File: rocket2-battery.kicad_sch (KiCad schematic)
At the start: 58 parts, among them J1 Conn_01x07, J2 SMA, J3 ARM Cortex Debug, P1 PAD_SMD, P2 PAD_SMD, P3 PAD_SMD, P4 PAD_SMD, P5 PAD_SMD, P6 PAD_SMD, P7 PAD_SMD, Q1 NMOS, Q2 NMOS, Q3 PMOS, Q4 PMOS, Q5 NMOS, Q6 NMOS, Q7 PMOS, Q8 PMOS, U1 3V3 LDO, Y1 16MHz

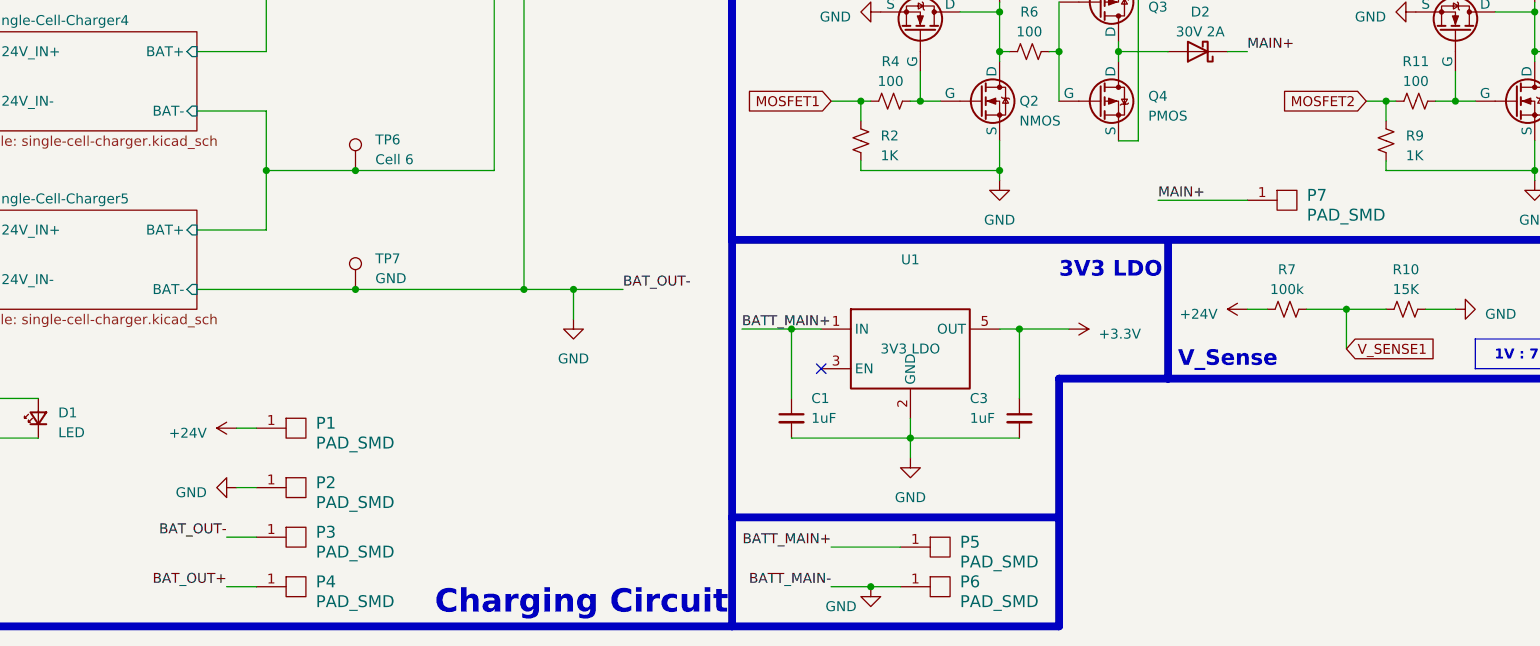
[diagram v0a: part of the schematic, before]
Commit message: Almost done routing
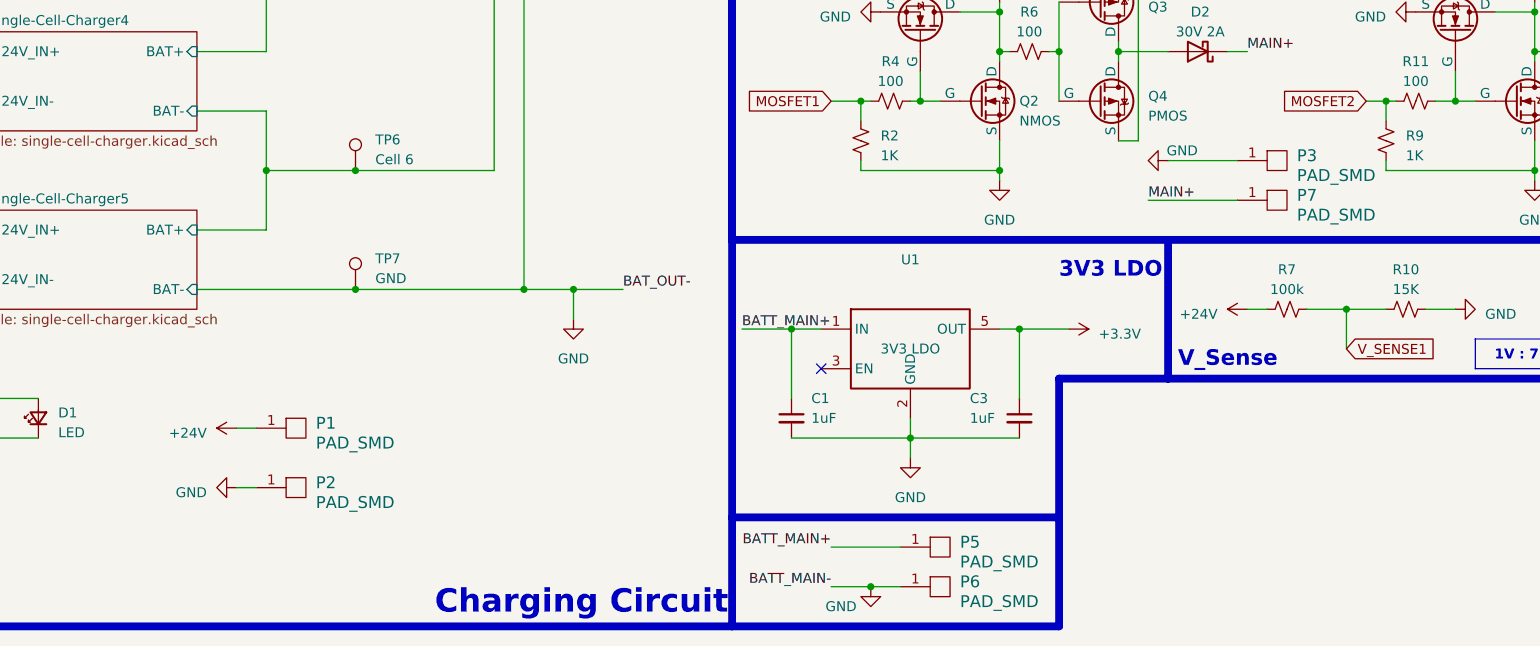
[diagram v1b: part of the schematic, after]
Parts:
- removed P4: PAD_SMD, TestPoint:TestPoint_Pad_2.0x2.0mm, symbol pkl_misc:PAD_SMD
- R8: footprint Resistor_SMD:R_0603_1608Metric -> Resistor_SMD:R_0603_1608Metric_Pad0.98x0.95mm_HandSolder
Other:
- moved on the sheet: P7
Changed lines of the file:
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@@
     (stroke (width 0) (type default))
   )
-  (wire (pts (xy 189.23 142.24) (xy 200.66 142.24))
+  (wire (pts (xy 187.96 142.24) (xy 199.39 142.24))
     (stroke (width 0) (type default))
   )
@@
     (stroke (width 0) (type default))
   )
-  (wire (pts (xy 69.85 185.42) (xy 73.66 185.42))
-    (stroke (width 0) (type default))
-  )
   (wire (pts (xy 255.27 95.25) (xy 257.81 95.25))
     (stroke (width 0) (type default))
@@
     (stroke (width 0) (type default))
   )
+  (wire (pts (xy 190.5 137.16) (xy 199.39 137.16))
+    (stroke (width 0) (type default))
+  )
   (wire (pts (xy 147.32 191.77) (xy 152.4 191.77))
     (stroke (width 0) (type default))
@@
     (stroke (width 0) (type default))
   )
-  (wire (pts (xy 69.85 191.77) (xy 73.66 191.77))
-    (stroke (width 0) (type default))
-  )
   (wire (pts (xy 208.28 156.21) (xy 213.36 156.21))
     (stroke (width 0) (type default))
@@
     (effects (font (size 1.27 1.27)) (justify left bottom))
   )
-  (label "MAIN+" (at 189.23 142.24 0) (fields_autoplaced)
+  (label "MAIN+" (at 187.96 142.24 0) (fields_autoplaced)
     (effects (font (size 1.27 1.27)) (justify left bottom))
   )
@@
     (effects (font (size 1.27 1.27)) (justify right bottom))
   )
-  (label "BAT_OUT-" (at 69.85 185.42 180) (fields_autoplaced)
-    (effects (font (size 1.27 1.27)) (justify right bottom))
-  )
   (label "BATT_MAIN+" (at 237.49 109.22 0) (fields_autoplaced)
     (effects (font (size 1.27 1.27)) (justify left bottom))
   )
-  (label "BAT_OUT+" (at 69.85 191.77 180) (fields_autoplaced)
-    (effects (font (size 1.27 1.27)) (justify right bottom))
-  )
   (label "BATT_MAIN+" (at 135.89 158.75 0) (fields_autoplaced)
     (effects (font (size 1.27 1.27)) (justify left bottom))
@@
     )
   )
+  (symbol (lib_id "power:GND") (at 190.5 137.16 270) (unit 1)
+    (in_bom yes) (on_board yes) (dnp no)
+    (property "Reference" "#PWR044" (at 184.15 137.16 0)
+      (effects (font (size 1.27 1.27)) hide)
+    )
+    (property "Value" "GND" (at 194.31 135.89 90)
+      (effects (font (size 1.27 1.27)) (justify right))
+    )
+    (property "Footprint" "" (at 190.5 137.16 0)
+      (effects (font (size 1.27 1.27)) hide)
+    )
+    (property "Datasheet" "" (at 190.5 137.16 0)
+      (effects (font (size 1.27 1.27)) hide)
+    )
+    (pin "1")
+    (instances
+      (project "rocket2-battery"
+        (path "/453543af-7e3c-49a0-a644-4bd49c4f86f8"
+          (reference "#PWR044") (unit 1)
+        )
+      )
+    )
+  )
   (symbol (lib_id "Device:LED_Small") (at 222.25 62.23 180) (unit 1)
     (in_bom yes) (on_board yes) (dnp no)
@@
     )
   )
-  (symbol (lib_id "pkl_misc:PAD_SMD") (at 78.74 191.77 0) (unit 1)
-    (in_bom yes) (on_board yes) (dnp no) (fields_autoplaced)
-    (property "Reference" "P4" (at 81.28 191.135 0)
-      (effects (font (size 1.524 1.524)) (justify left))
-    )
-    (property "Value" "PAD_SMD" (at 81.28 193.675 0)
-      (effects (font (size 1.524 1.524)) (justify left))
-    )
-    (property "Footprint" "TestPoint:TestPoint_Pad_2.0x2.0mm" (at 78.74 198.12 0)
-      (effects (font (size 1.524 1.524)) hide)
-    )
-    (property "Datasheet" "~" (at 78.74 195.58 0)
-      (effects (font (size 1.524 1.524)))
-    )
-    (property "Manufacturer" "Generic" (at 78.74 191.77 0)
-      (effects (font (size 1.27 1.27)) hide)
-    )
-    (pin "1")
-    (instances
-      (project "rocket2-battery"
-        (path "/453543af-7e3c-49a0-a644-4bd49c4f86f8"
-          (reference "P4") (unit 1)
-        )
-      )
-    )
-  )
   (symbol (lib_id "Device:C_Small") (at 210.82 22.86 0) (unit 1)
     (in_bom yes) (on_board yes) (dnp no)
@@
     )
   )
-  (symbol (lib_id "pkl_misc:PAD_SMD") (at 78.74 185.42 0) (unit 1)
-    (in_bom yes) (on_board yes) (dnp no) (fields_autoplaced)
-    (property "Reference" "P3" (at 81.28 184.785 0)
-      (effects (font (size 1.524 1.524)) (justify left))
-    )
-    (property "Value" "PAD_SMD" (at 81.28 187.325 0)
-      (effects (font (size 1.524 1.524)) (justify left))
-    )
-    (property "Footprint" "TestPoint:TestPoint_Pad_2.0x2.0mm" (at 78.74 191.77 0)
-      (effects (font (size 1.524 1.524)) hide)
-    )
-    (property "Datasheet" "~" (at 78.74 189.23 0)
-      (effects (font (size 1.524 1.524)))
-    )
-    (property "Manufacturer" "Generic" (at 78.74 185.42 0)
-      (effects (font (size 1.27 1.27)) hide)
-    )
-    (pin "1")
-    (instances
-      (project "rocket2-battery"
-        (path "/453543af-7e3c-49a0-a644-4bd49c4f86f8"
-          (reference "P3") (unit 1)
-        )
-      )
-    )
-  )
   (symbol (lib_id "power:+3.3V") (at 275.59 58.42 0) (unit 1)
     (in_bom yes) (on_board yes) (dnp no)
@@
     )
   )
+  (symbol (lib_id "pkl_misc:PAD_SMD") (at 204.47 137.16 0) (unit 1)
+    (in_bom yes) (on_board yes) (dnp no) (fields_autoplaced)
+    (property "Reference" "P3" (at 207.01 136.525 0)
+      (effects (font (size 1.524 1.524)) (justify left))
+    )
+    (property "Value" "PAD_SMD" (at 207.01 139.065 0)
+      (effects (font (size 1.524 1.524)) (justify left))
+    )
+    (property "Footprint" "TestPoint:TestPoint_Pad_2.0x2.0mm" (at 204.47 143.51 0)
+      (effects (font (size 1.524 1.524)) hide)
+    )
+    (property "Datasheet" "~" (at 204.47 140.97 0)
+      (effects (font (size 1.524 1.524)))
+    )
+    (property "Manufacturer" "Generic" (at 204.47 137.16 0)
+      (effects (font (size 1.27 1.27)) hide)
+    )
+    (pin "1")
+    (instances
+      (project "rocket2-battery"
+        (path "/453543af-7e3c-49a0-a644-4bd49c4f86f8"
+          (reference "P3") (unit 1)
+        )
+      )
+    )
+  )
   (symbol (lib_id "Connector:Conn_Coaxial") (at 232.41 93.98 90) (mirror x) (unit 1)
     (in_bom yes) (on_board yes) (dnp no)
@@
     )
   )
-  (symbol (lib_id "pkl_misc:PAD_SMD") (at 205.74 142.24 0) (unit 1)
+  (symbol (lib_id "pkl_misc:PAD_SMD") (at 204.47 142.24 0) (unit 1)
     (in_bom yes) (on_board yes) (dnp no) (fields_autoplaced)
-    (property "Reference" "P7" (at 208.28 141.605 0)
+    (property "Reference" "P7" (at 207.01 141.605 0)
       (effects (font (size 1.524 1.524)) (justify left))
     )
-    (property "Value" "PAD_SMD" (at 208.28 144.145 0)
+    (property "Value" "PAD_SMD" (at 207.01 144.145 0)
       (effects (font (size 1.524 1.524)) (justify left))
     )
-    (property "Footprint" "TestPoint:TestPoint_Pad_2.0x2.0mm" (at 205.74 148.59 0)
+    (property "Footprint" "TestPoint:TestPoint_Pad_2.0x2.0mm" (at 204.47 148.59 0)
       (effects (font (size 1.524 1.524)) hide)
     )
-    (property "Datasheet" "~" (at 205.74 146.05 0)
+    (property "Datasheet" "~" (at 204.47 146.05 0)
       (effects (font (size 1.524 1.524)))
     )
-    (property "Manufacturer" "Generic" (at 205.74 142.24 0)
+    (property "Manufacturer" "Generic" (at 204.47 142.24 0)
       (effects (font (size 1.27 1.27)) hide)
     )
@@
       (effects (font (size 1.27 1.27)))
     )
-    (property "Footprint" "Resistor_SMD:R_0603_1608Metric" (at 213.36 62.23 0)
+    (property "Footprint" "Resistor_SMD:R_0603_1608Metric_Pad0.98x0.95mm_HandSolder" (at 213.36 62.23 0)
       (effects (font (size 1.27 1.27)) hide)
     )

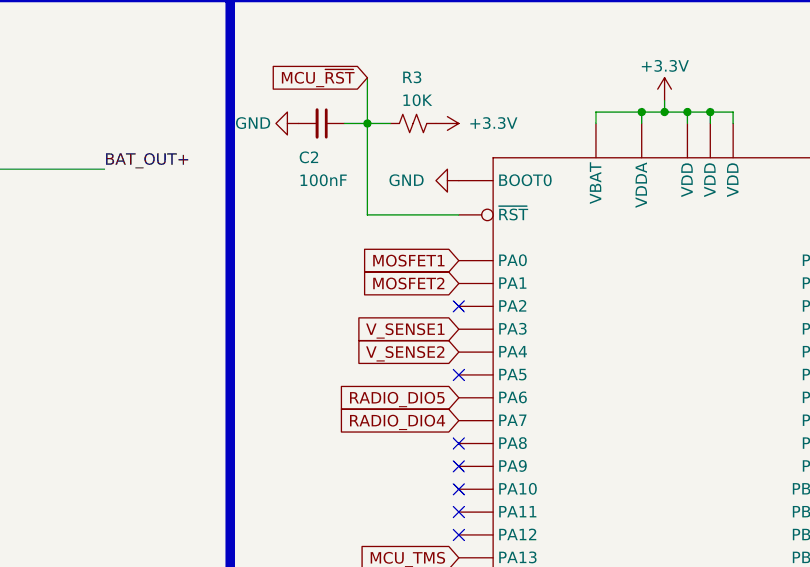
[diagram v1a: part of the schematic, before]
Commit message: Finished most of layout
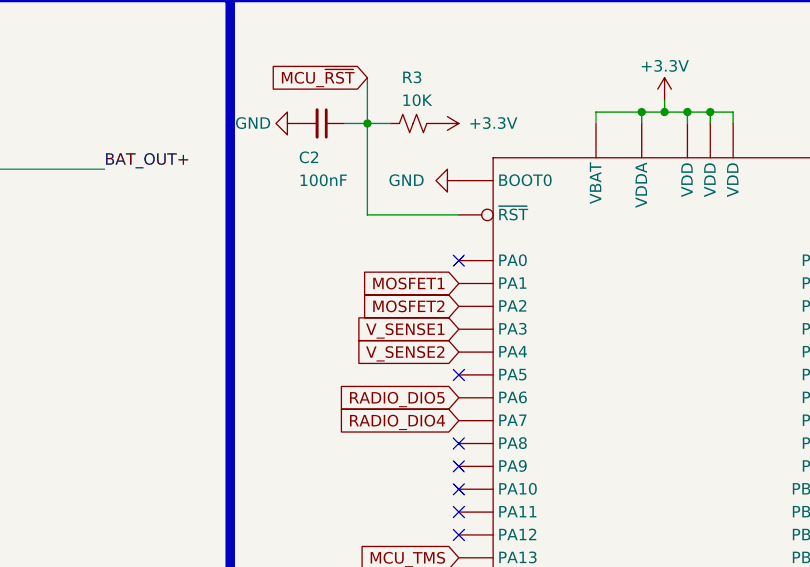
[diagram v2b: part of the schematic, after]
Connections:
- net MOSFET1: now also U2.11 (PA1); no longer U2.10 (PA0)
- net MOSFET2: now also U2.12 (PA2); no longer U2.11 (PA1)
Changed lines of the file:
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@@
   (no_connect (at 160.02 83.82))
   (no_connect (at 160.02 72.39))
-  (no_connect (at 160.02 46.99))
+  (no_connect (at 160.02 41.91))
   (no_connect (at 160.02 88.9))
   (no_connect (at 160.02 62.23))
@@
     )
   )
-  (global_label "MOSFET1" (shape input) (at 160.02 41.91 180) (fields_autoplaced)
-    (effects (font (size 1.27 1.27)) (justify right))
-    (property "Intersheetrefs" "${INTERSHEET_REFS}" (at 148.7081 41.91 0)
+  (global_label "MOSFET1" (shape input) (at 160.02 44.45 180) (fields_autoplaced)
+    (effects (font (size 1.27 1.27)) (justify right))
+    (property "Intersheetrefs" "${INTERSHEET_REFS}" (at 148.7081 44.45 0)
       (effects (font (size 1.27 1.27)) (justify right) hide)
     )
@@
     )
   )
-  (global_label "MOSFET2" (shape input) (at 160.02 44.45 180) (fields_autoplaced)
-    (effects (font (size 1.27 1.27)) (justify right))
-    (property "Intersheetrefs" "${INTERSHEET_REFS}" (at 148.7081 44.45 0)
-      (effects (font (size 1.27 1.27)) (justify right) hide)
-    )
+  (global_label "MOSFET2" (shape input) (at 160.02 46.99 180) (fields_autoplaced)
+    (effects (font (size 1.27 1.27)) (justify right))
+    (property "Intersheetrefs" "${INTERSHEET_REFS}" (at 148.7081 46.99 0)
+      (effects (font (size 1.27 1.27)) (justify right) hide)
+    )
